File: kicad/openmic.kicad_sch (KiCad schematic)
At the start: 0 parts

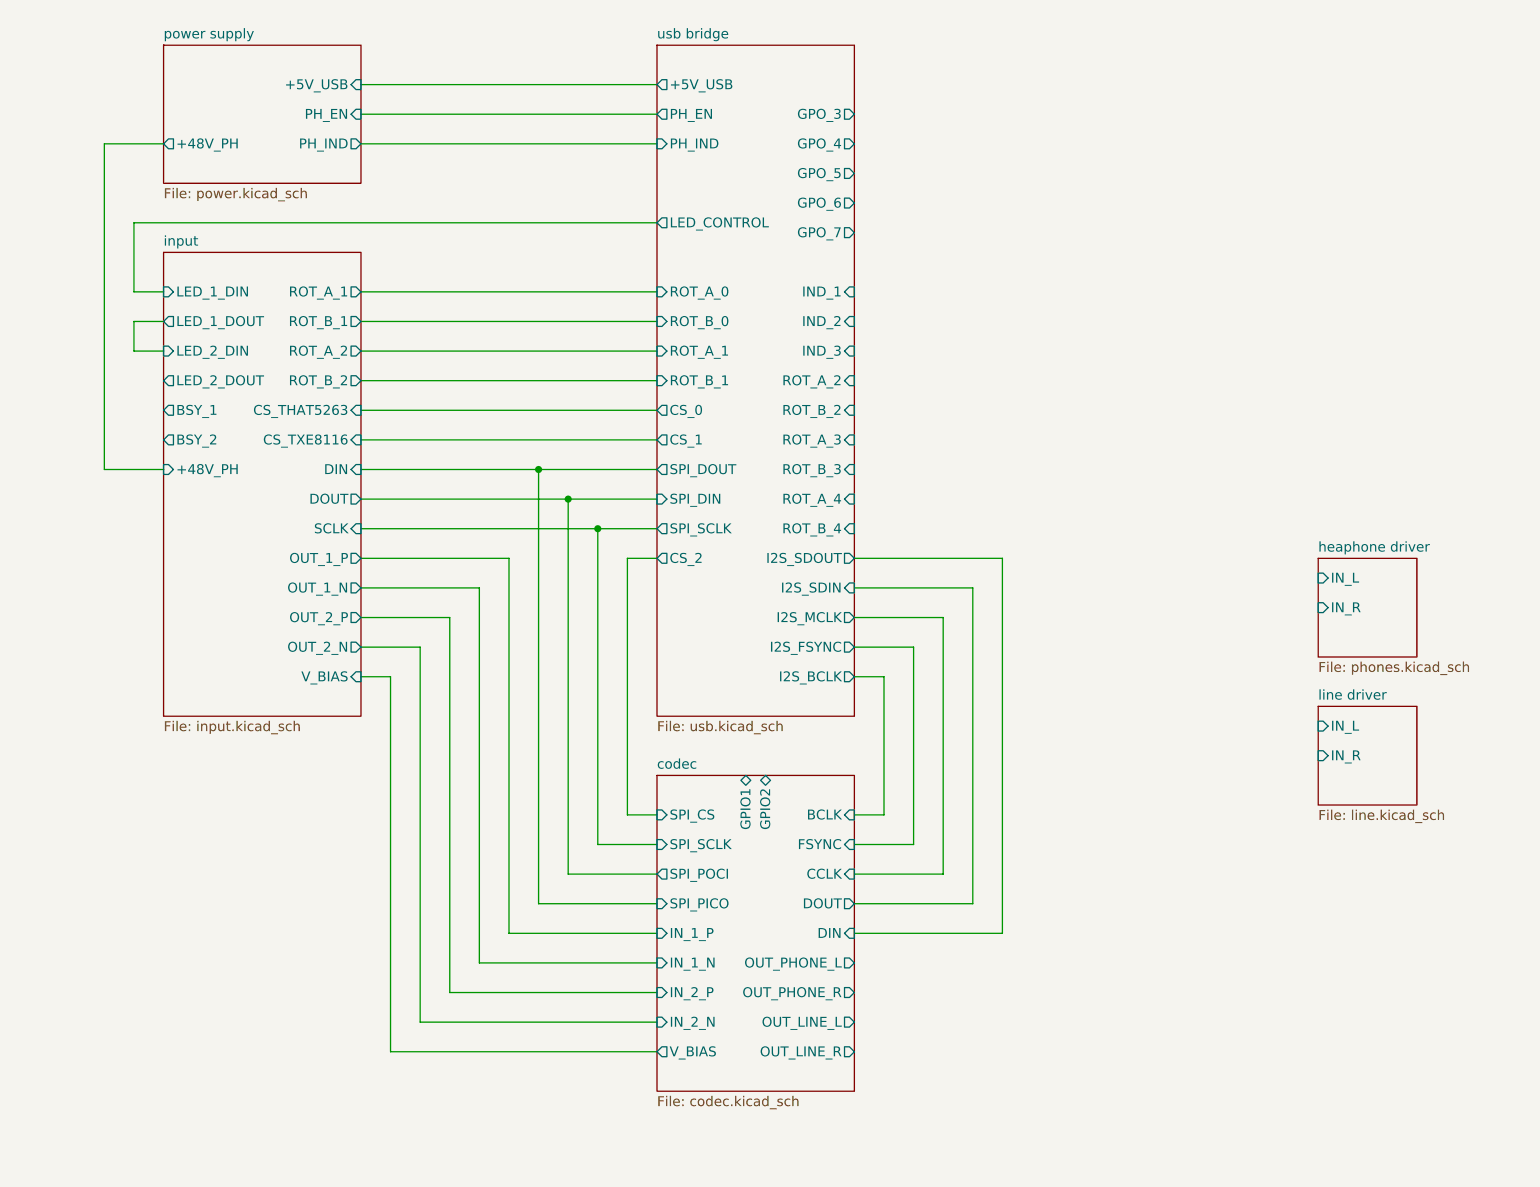
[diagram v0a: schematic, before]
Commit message: phones out
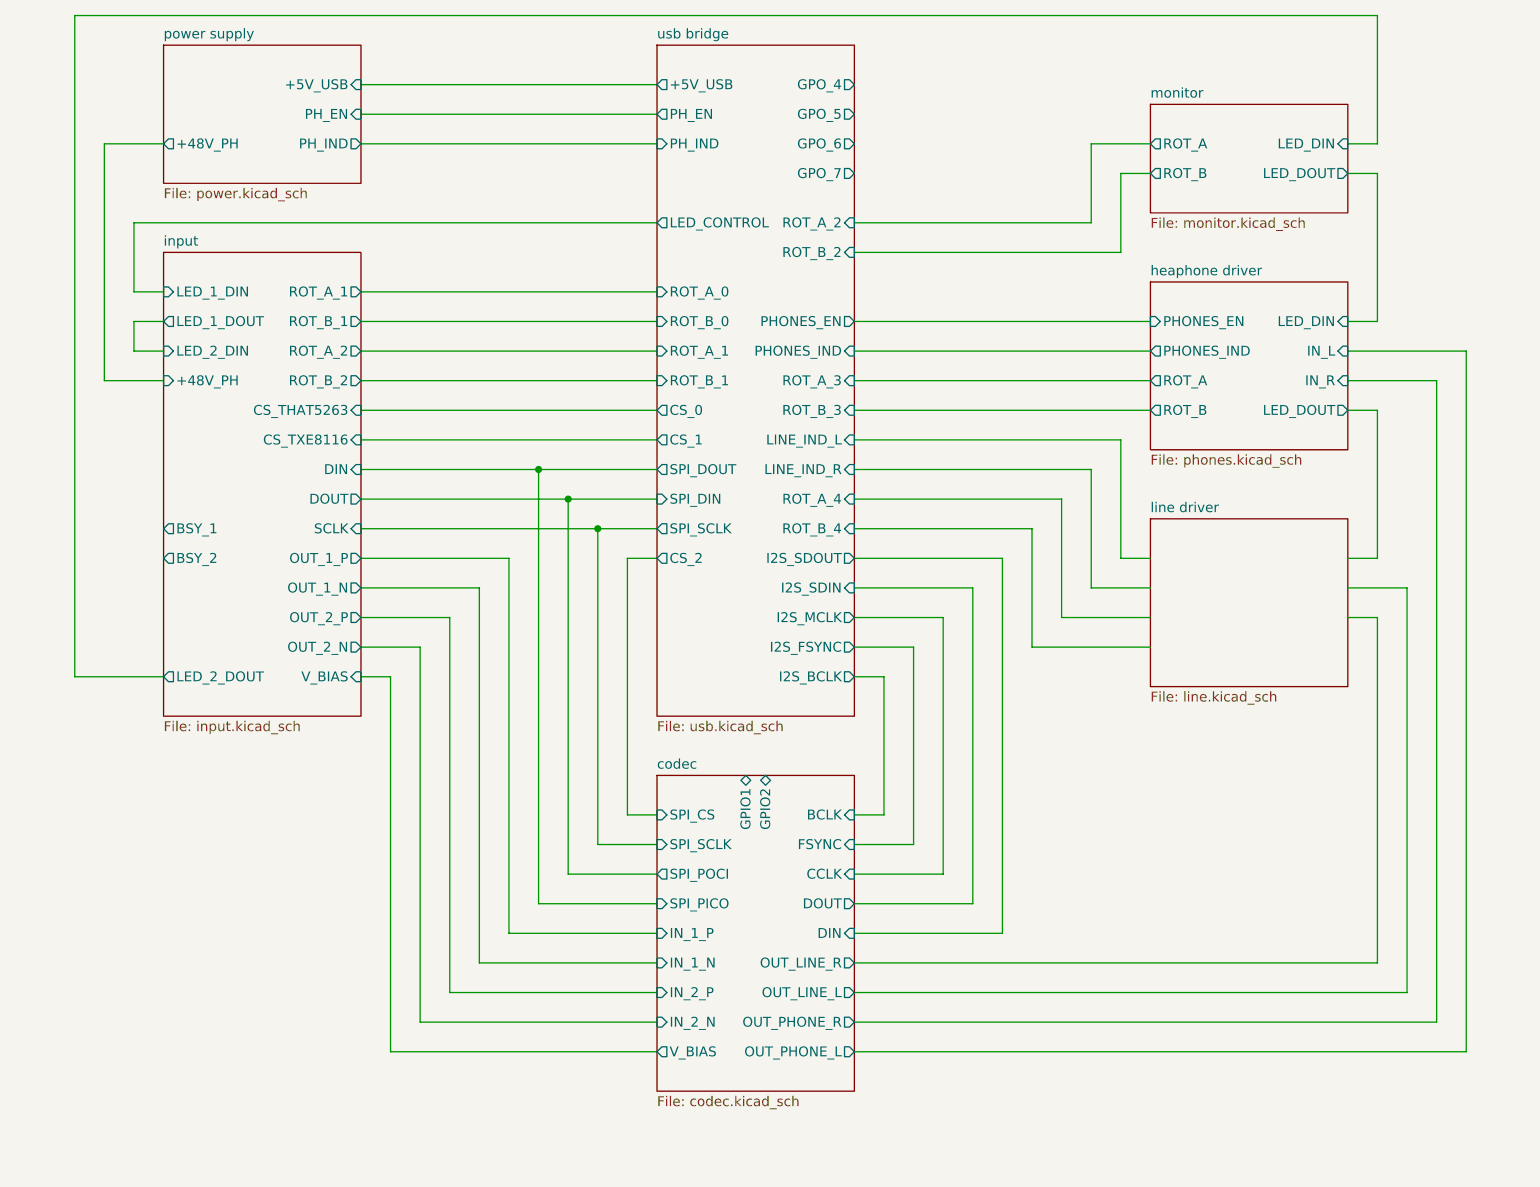
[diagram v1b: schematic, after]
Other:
- added sheet monitor (monitor.kicad_sch)
- sheet heaphone driver ports: added LED_DIN, LED_DOUT, PHONES_EN, PHONES_IND, ROT_A, ROT_B; removed none
- sheet line driver ports: added none; removed IN_L, IN_R
- sheet usb bridge ports: added LINE_IND_L, LINE_IND_R, PHONES_EN, PHONES_IND; removed GPO_3, IND_1, IND_2, IND_3

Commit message: line out
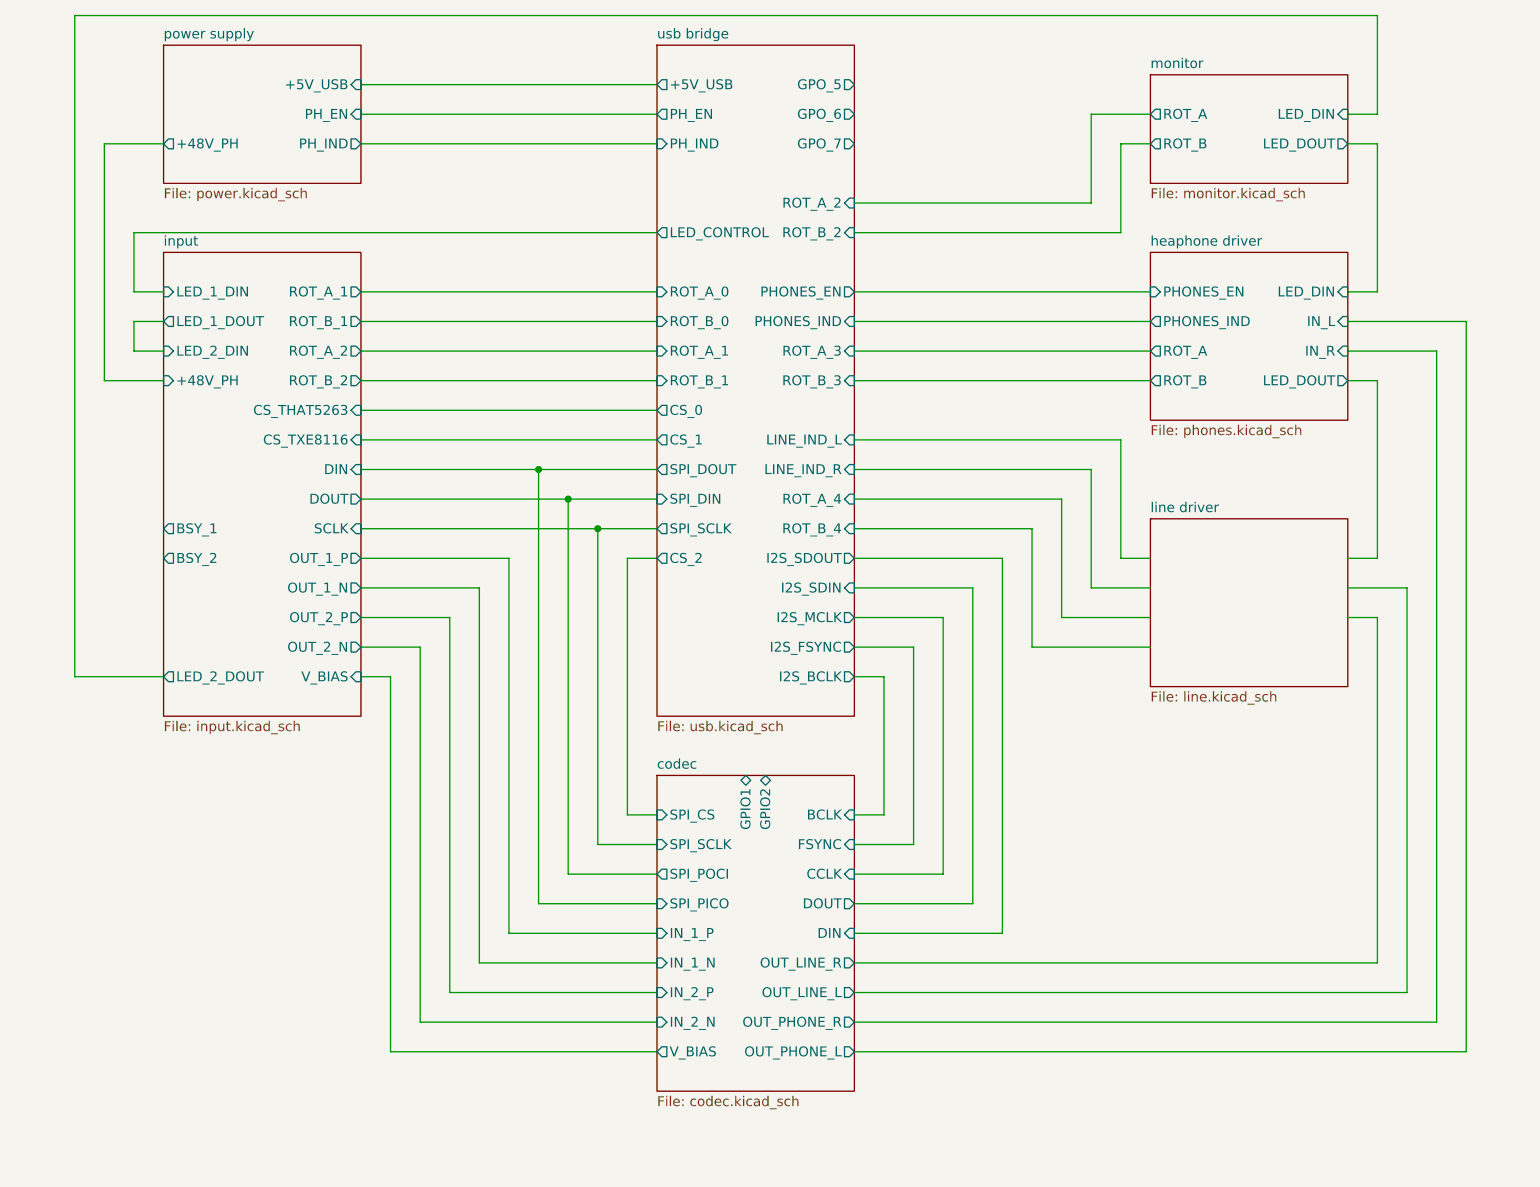
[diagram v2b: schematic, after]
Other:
- sheet usb bridge ports: added none; removed GPO_4

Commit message: input enable
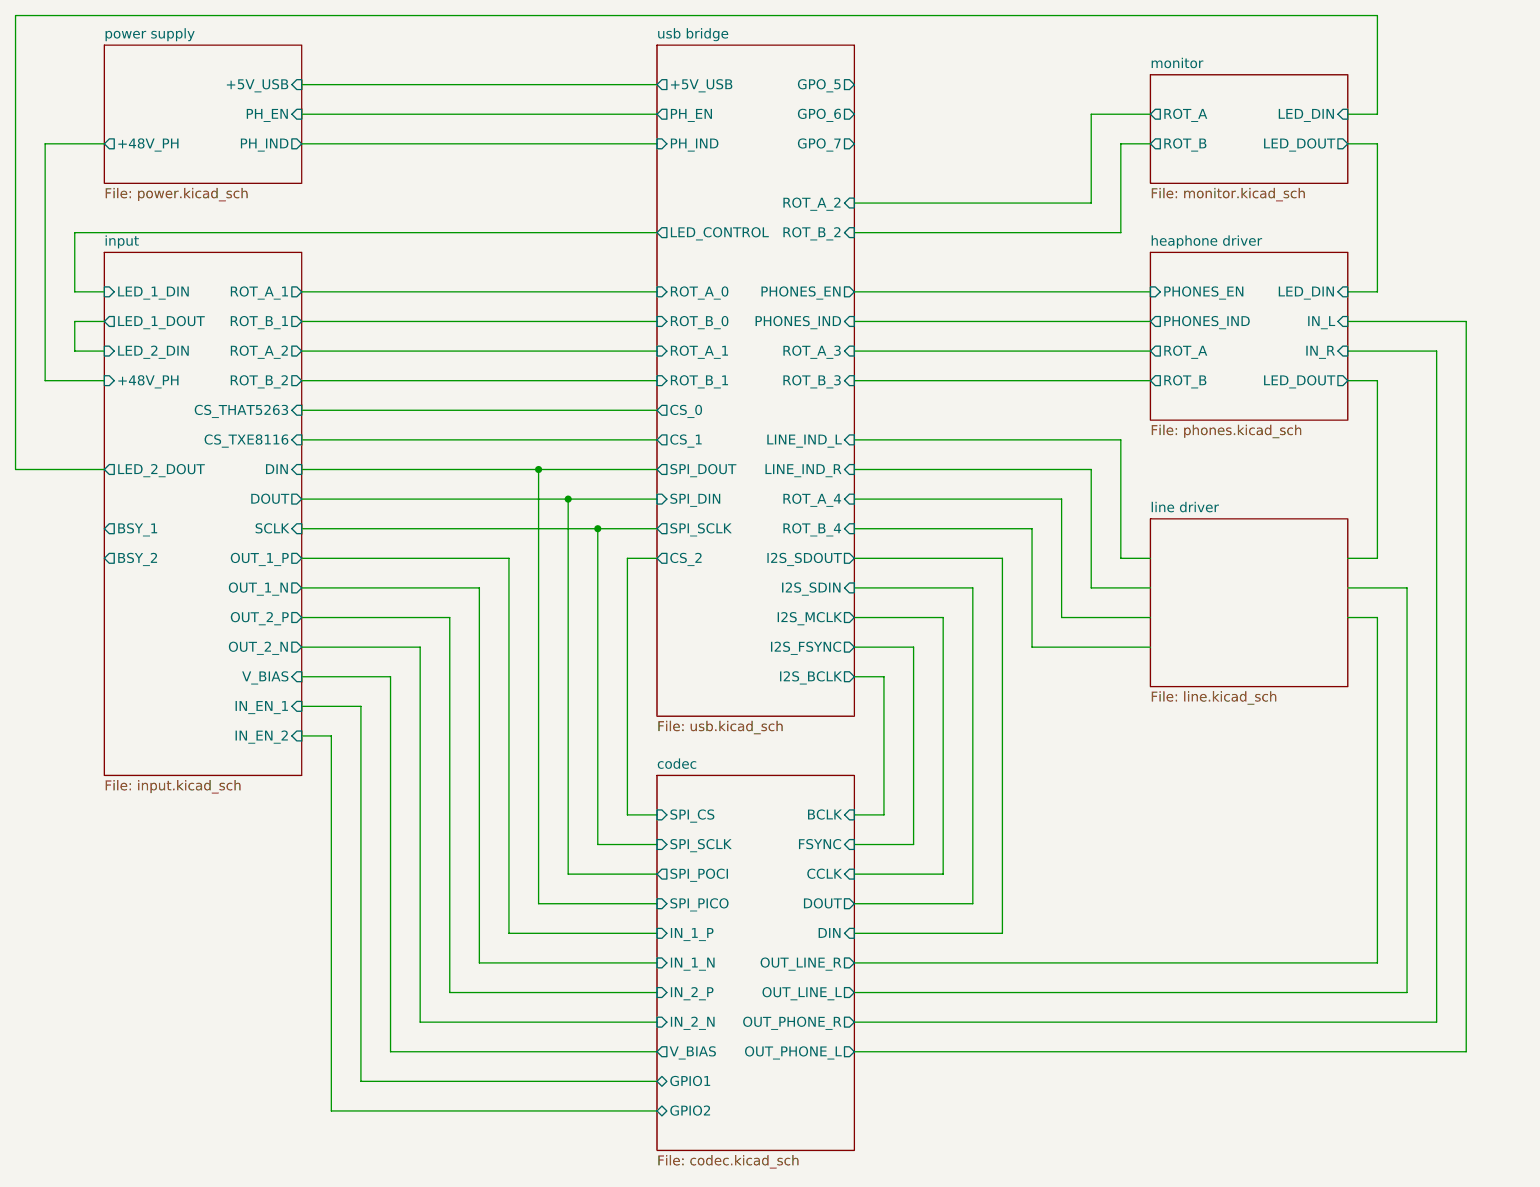
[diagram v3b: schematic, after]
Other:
- sheet input ports: added IN_EN_1, IN_EN_2; removed none
